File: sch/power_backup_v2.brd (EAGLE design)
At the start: 56 x 33.5 mm, 38 parts, among them IC1 78L05SMD, IC2 ACS712-LC, K1 DS2Y-S-DC48V, K2 HFD2/003, T1 BC847, T2 BC847, T3 BC847, T4 BC847

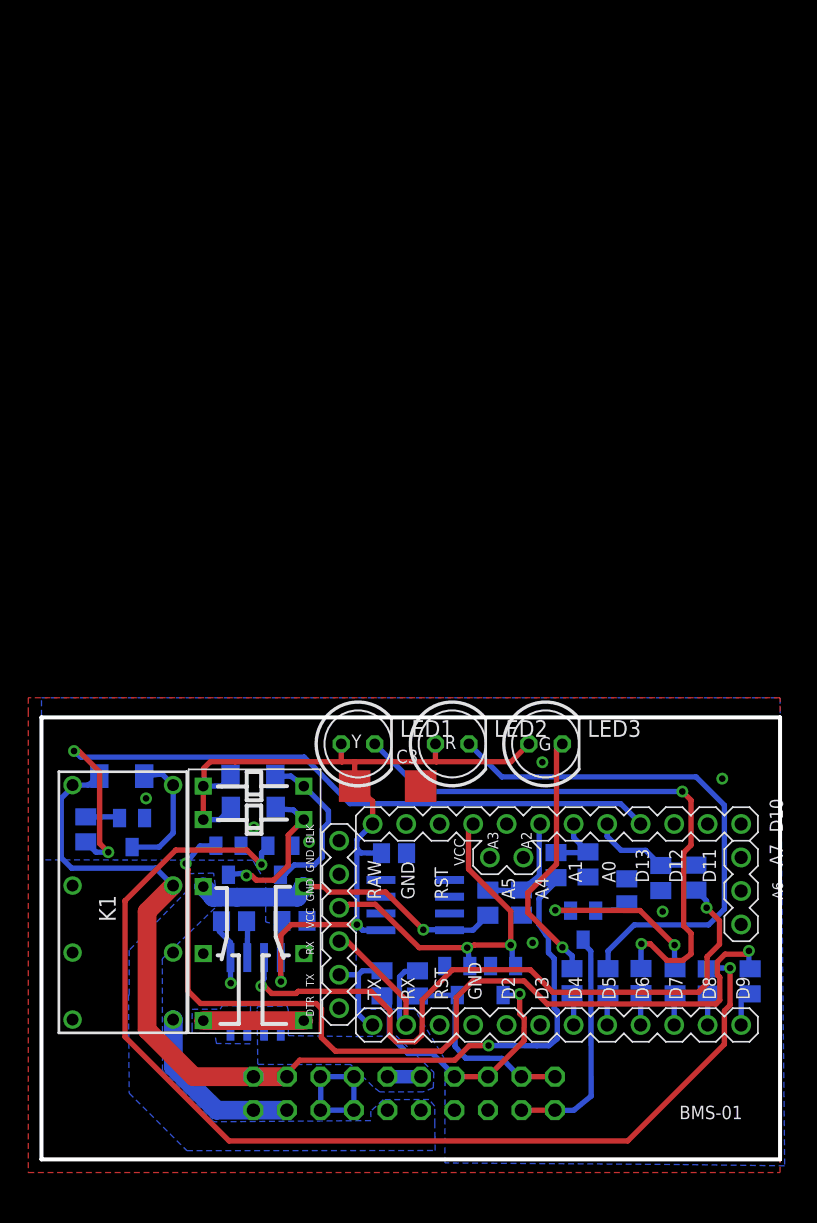
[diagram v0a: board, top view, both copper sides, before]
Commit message: version 2
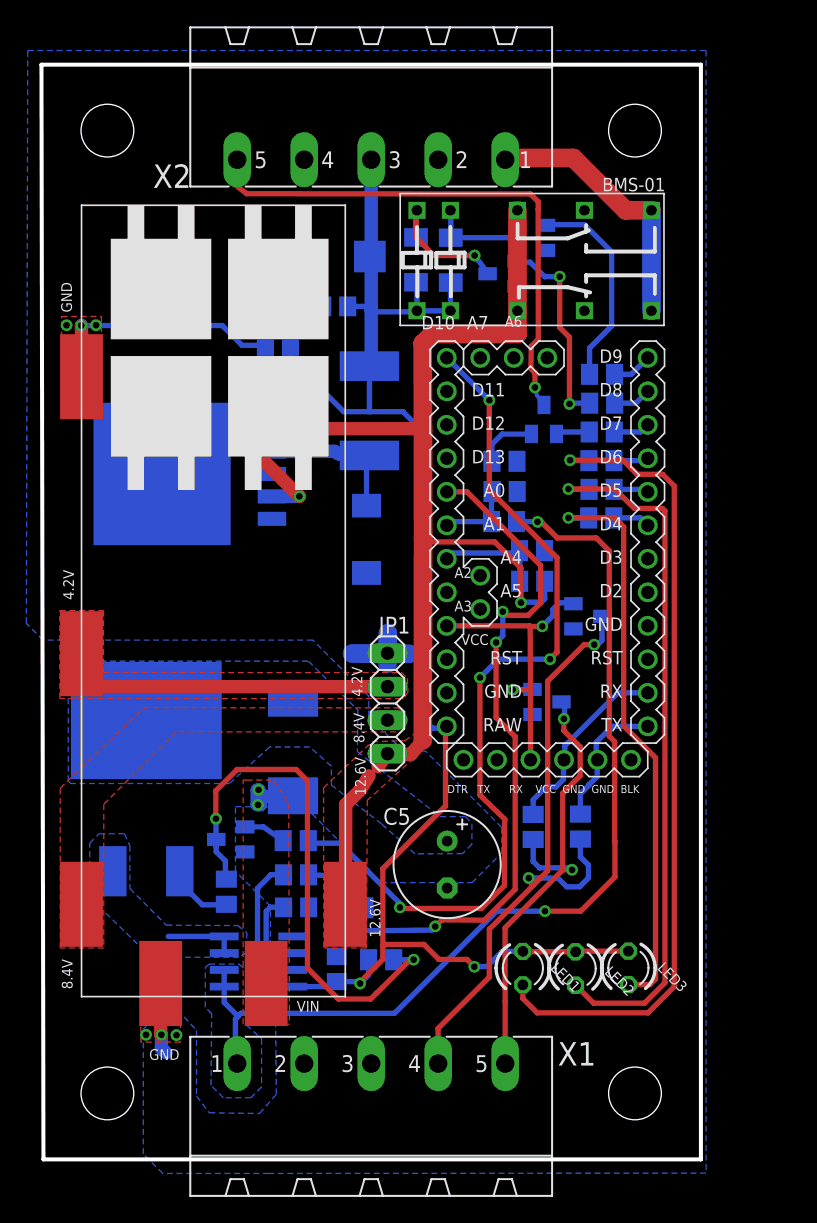
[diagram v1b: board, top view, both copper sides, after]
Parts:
- removed IC1: 78L05SMD, linear:SO08
- removed K1: DS2Y-S-DC48V, relay:DS2Y
- removed SV1: (no value), con-lstb:MA10-2
- added C5: (no value), rcl:E3,5-8
- added D6: (no value), eagle-ltspice:DIODE_SMC
- added IC3: LM2576-ADJ, linear:TO263-5
- added JP1: (no value), pinhead:1X04
- added L1: 220u, inductor-neosid:MS85
- added Q2: IRF3704S, transistor-power:D2PACK
- added R13, R18: 1k, rcl:M0805
- added R19: 6K2, rcl:M0805
- added R20: 2K, rcl:M0805
- added U$1: BALANCER, balancer20a:BALANCER
- added X1, X2: MSTBA5, con-phoenix-508:MSTBA5
- D3: value PMLL4150 -> (none); device diode:SOD80C -> diode:DO214AA
- IC2: value ACS712-LC -> ACS712-5A
- LED1, LED2, LED3: device led:LED5MM -> led:LED3MM
- R12: value 560 -> 1k
- moved T3 52.5 mm to (37.2, 69.9), turned to 270 degrees
- moved T2 47.5 mm to (34.9, 67.1), turned to 270 degrees
- moved R10 47.4 mm to (42.5, 59.5), turned to 180 degrees
- moved R11 44.6 mm to (42.5, 57.3), turned to 180 degrees
- moved D2 44.2 mm to (31.0, 68.2), turned to 90 degrees
- moved K2 44.1 mm to (27.2, 73.2), turned to 270 degrees
- moved R7 42.0 mm to (42.5, 55.2), turned to 180 degrees
- moved C4 41.7 mm to (22.3, 64.7), turned to 0 degrees
- moved D1 41.1 mm to (28.4, 68.2), turned to 90 degrees
- moved C3 40.3 mm to (22.4, 68.4), flipped to the bottom
- moved R1 39.6 mm to (42.5, 53.0), turned to 180 degrees
- moved T1 38.5 mm to (38.1, 56.1), turned to 0 degrees
- moved R2 37.3 mm to (42.5, 50.8), turned to 180 degrees
- moved R3 35.2 mm to (42.4, 48.6), turned to 180 degrees
- moved R6 33.9 mm to (35.1, 52.9), turned to 0 degrees
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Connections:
- removed net CON_VBATP: IC1.8, K2.P$13, K2.P$4, R9.2, SV1.10, SV1.12
- removed net S_REL_IN: ARDUINO1.D13, R12.2
- removed net VOUT: IC2.3, IC2.4, K2.P$8, K2.P$9
- new net BAT12V: IC3.1, JP1.1, K2.P$13, K2.P$4, R9.2, U$1.12V
- new net BAT4V: JP1.3, U$1.4V
- new net BAT8V: JP1.2, U$1.8V
- new net N$16: R18.1, T4.1
- new net N$22: D3.C, IC3.2, L1.1
- new net N$23: IC3.4, R19.2, R20.1
- new net N$4: C5.+, D6.A, Q2.2
- new net PWRP: IC2.3, IC2.4, Q2.3
- new net S_PWR_REG: ARDUINO1.D10, R18.2
- net +5V: now also L1.2, R12.1, R19.1, X2.3; no longer IC1.1
- net CON_ERROR_OC: now also X2.5; no longer SV1.18, SV1.20
- net CON_PWR2P: now also D6.C, U$1.VIN; no longer K1.9, SV1.2, SV1.4
- net CON_PWRP: now also IC2.1, IC2.2, X1.1; no longer D3.C, K1.1, K1.13, SV1.1, SV1.3
- net CON_RX: now also X1.5; no longer SV1.17, SV1.19
- net CON_TX: now also X1.4; no longer SV1.13, SV1.15
- net CON_VOUT: now also K2.P$8, K2.P$9, X2.1; no longer IC2.1, IC2.2, SV1.11, SV1.9
- net GND: now also C5.-, D3.A, IC3.3, IC3.5, IC3.6, JP1.4, R20.2, U$1.0V, U$1.GND, X1.2, X1.3, X2.2, X2.4; no longer IC1.2, IC1.3, IC1.6, IC1.7, SV1.14, SV1.16, SV1.5, SV1.6, SV1.7, SV1.8
- net N$10: now also R12.2, R13.2, T4.3; no longer R12.1, T4.1
- net N$11: now also Q2.1, R13.1; no longer D3.A, K1.16, T4.3
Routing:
- net BAT12V: track 0.00 -> 88.0 mm, vias 0 -> 2
- net N$9: track 83.7 -> 15.6 mm
- net S_PWR_REG: track 0.00 -> 66.9 mm, vias 0 -> 4
- net S_REL_IN: track 56.3 -> 0.00 mm, vias 2 -> 0
- net N$8: track 68.1 -> 15.8 mm, vias 2 -> 0
- net +5V: track 69.1 -> 120.7 mm
- net S_IOUT: track 8.60 -> 57.8 mm, vias 0 -> 3
- net N$13: track 52.0 -> 11.3 mm, vias 2 -> 0
- net N$10: track 2.60 -> 41.5 mm, vias 0 -> 2
- net CON_TX: track 20.9 -> 48.7 mm, vias 1 -> 2
- net BAT4V: track 0.00 -> 25.7 mm
- net CON_VBATP: track 24.3 -> 0.00 mm, vias 1 -> 0
- net N$3: track 19.5 -> 43.5 mm
- net CON_ERROR_OC: track 17.8 -> 41.4 mm, vias 0 -> 1
- net CON_RX: track 15.5 -> 36.1 mm, vias 0 -> 2
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- added copper zone on layer 1, net BAT12V
- added copper zone on layer 1, net BAT4V
- added copper zone on layer 1, net BAT8V
- added copper zone on layer 1, net CON_PWR2P
- added copper zone on layer 16, net CON_PWRP
- added copper zone on layer 16, net N$4
- added copper zone on layer 16, net PWRP
- removed copper zone on layer 16, net CON_VBATP
- removed copper zone on layer 16, net CON_VOUT
- removed copper zone on layer 16, net VOUT
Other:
- board size 56 x 33.5 mm -> 50 x 83 mm
- board text added: "12.6V"
- board text added: "4.2V"
- board text added: "8.4V"
- board text added: "GND"
- board text added: "VIN"
- board text removed: "G"
- board text removed: "R"
- board text removed: "Y"
